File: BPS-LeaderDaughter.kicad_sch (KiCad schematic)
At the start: 10 parts, among them J1 DaughterConnector, J2 DaughterConnector

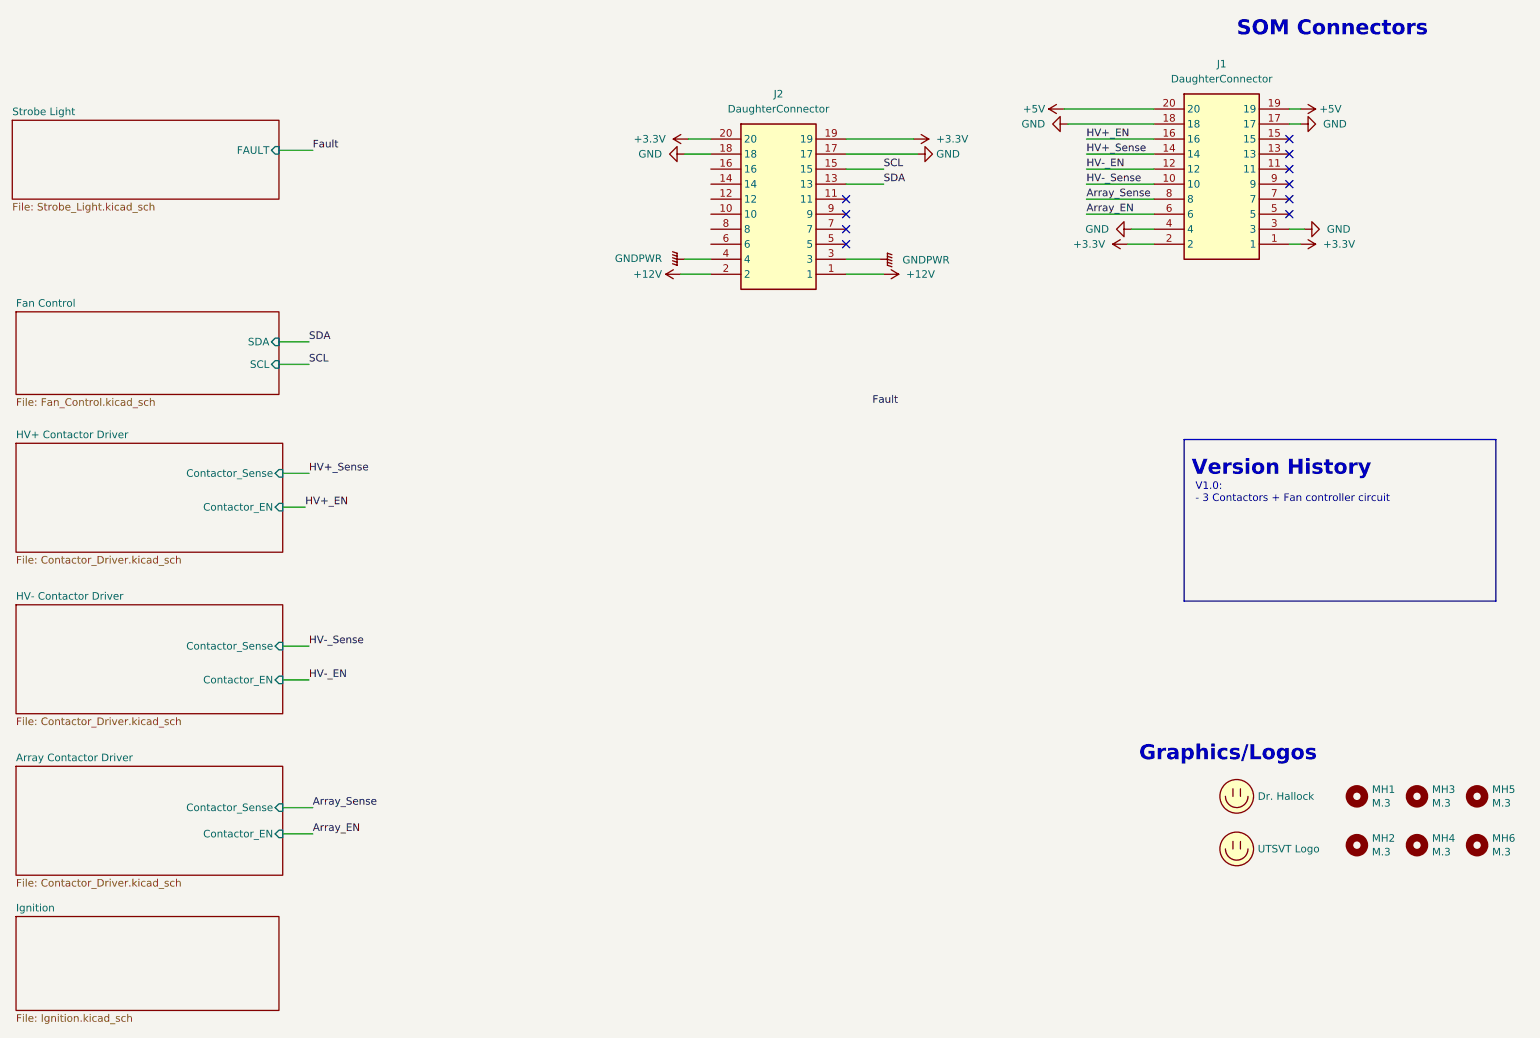
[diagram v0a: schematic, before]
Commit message: Restructed main sheet
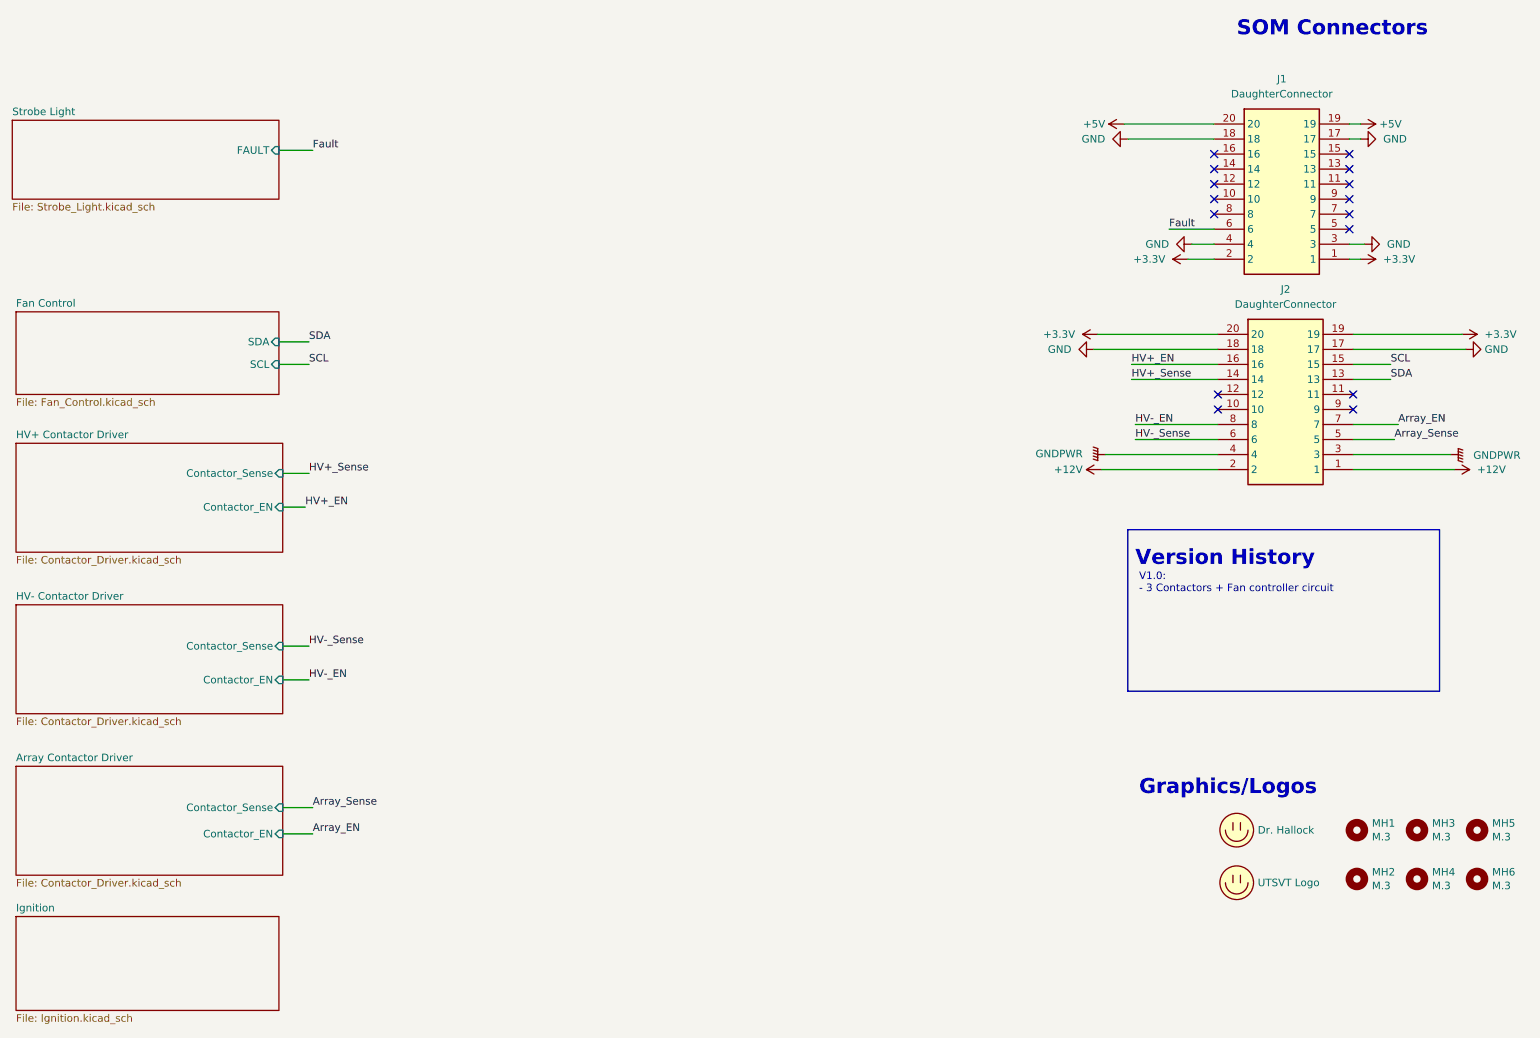
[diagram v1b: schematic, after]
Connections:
- net Array_EN: now also J2.7; no longer J1.6
- net Array_Sense: now also J2.5; no longer J1.8
- net Fault: now also J1.6
- net HV+_EN: now also J2.16; no longer J1.16
- net HV+_Sense: now also J2.14; no longer J1.14
- net HV-_EN: now also J2.8; no longer J1.12
- net HV-_Sense: now also J2.6; no longer J1.10
- no-connect marks 10 -> 15
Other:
- moved on the sheet: J1, J2, MH1, MH2, MH3, MH4, MH5, MH6
